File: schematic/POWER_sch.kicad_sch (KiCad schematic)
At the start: 24 parts, among them J4 10118194-0001LF, J5 PW_Conn, J6 PwSelectPin, J7 Power_conn, U4 LD39050PU33R, U5 L7805CDT-TR

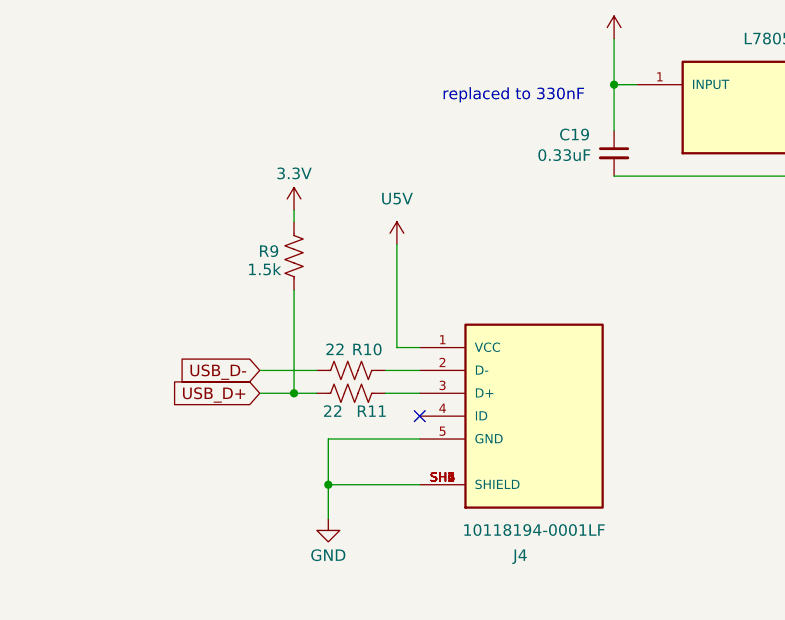
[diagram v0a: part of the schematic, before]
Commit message: Update README(schematic)
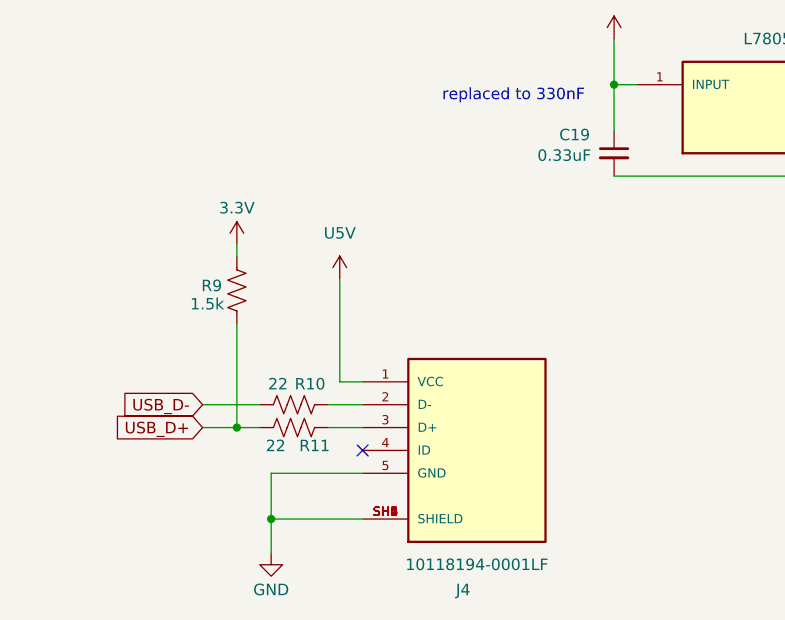
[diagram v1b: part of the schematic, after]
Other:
- moved on the sheet: J4, R10, R11, R9
